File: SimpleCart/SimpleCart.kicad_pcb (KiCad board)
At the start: 2 copper layers, 90 x 56.8 mm, 9 parts, among them J1 CommanderX16Expansion Alt, U1 SST39SF040, U2 74HCT00, U3 74HCT138

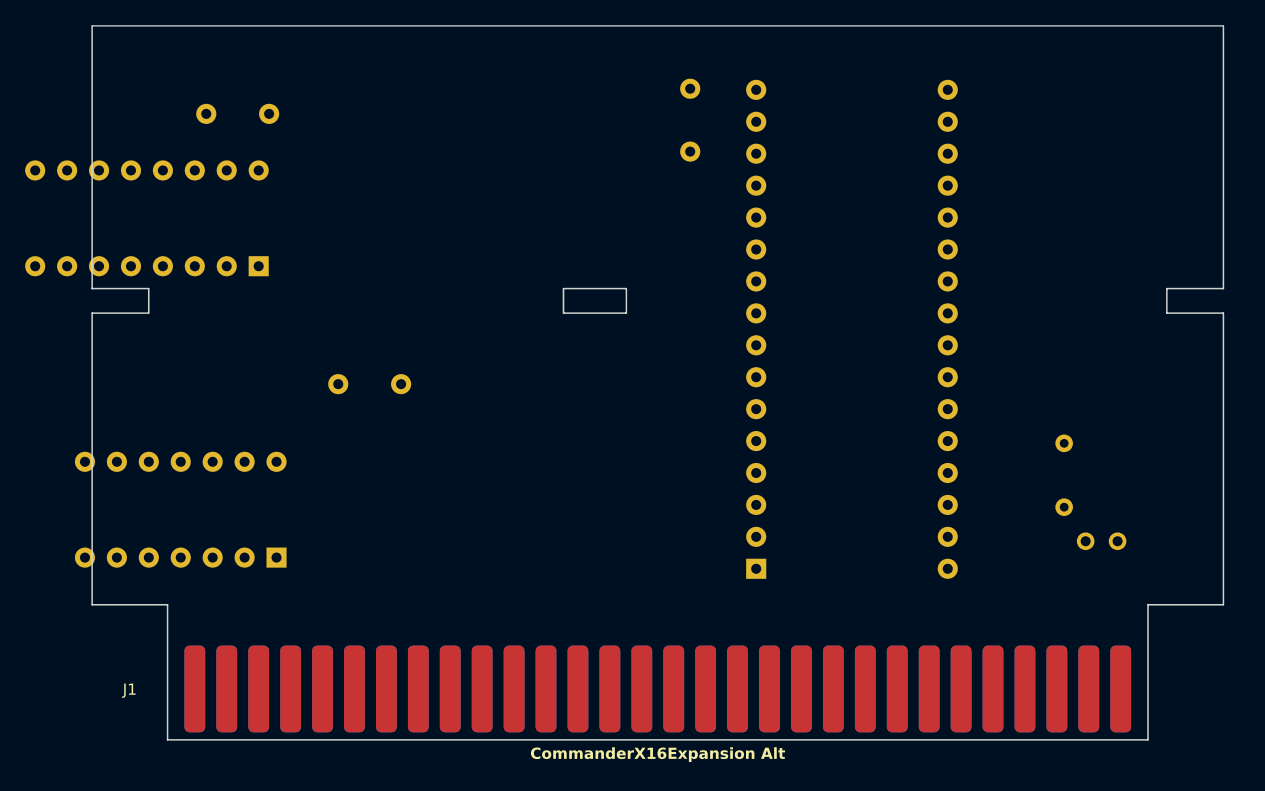
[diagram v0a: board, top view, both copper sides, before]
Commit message: BOM, fully routed
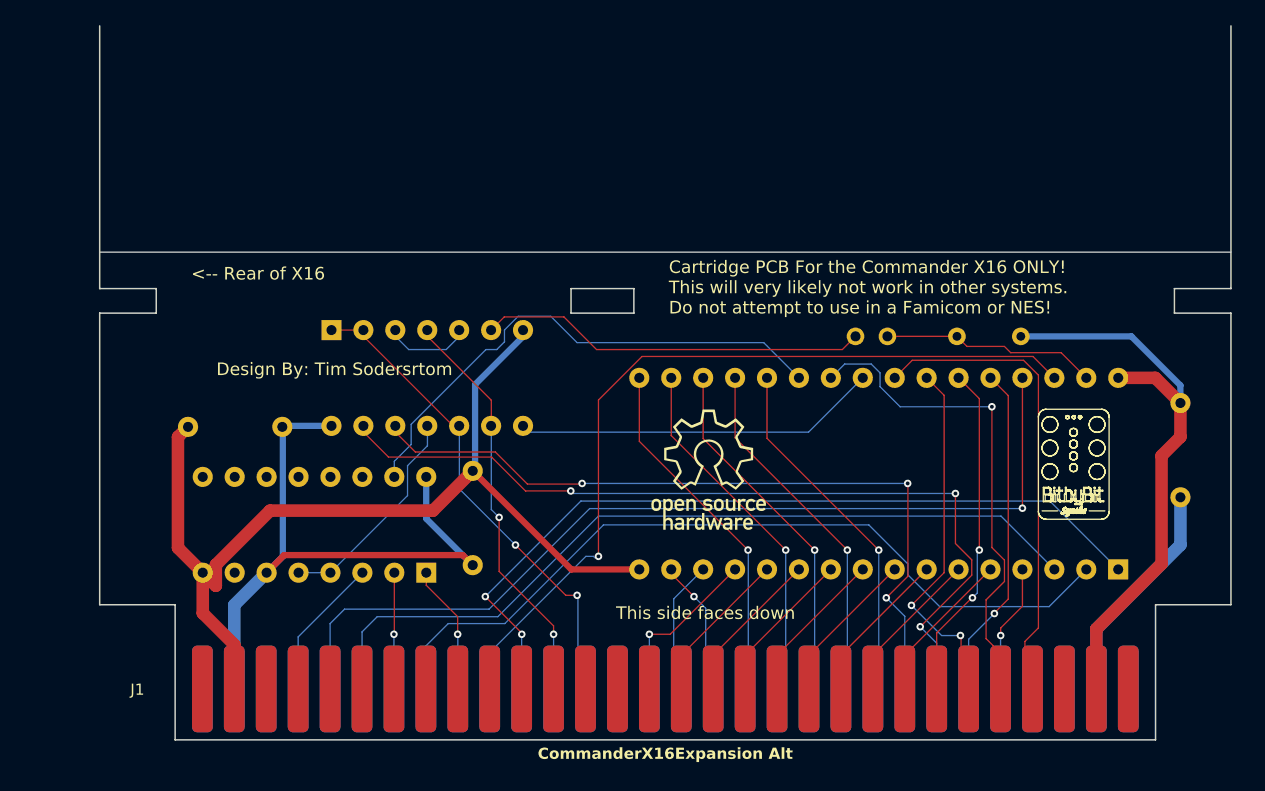
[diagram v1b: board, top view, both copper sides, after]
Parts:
- C1, C2, C3: value C -> 100nF; footprint Capacitor_THT:C_Disc_D5.0mm_W2.5mm_P5.00mm -> Capacitor_THT:C_Axial_L3.8mm_D2.6mm_P7.50mm_Horizontal
- JP1: value Jumper_2_Bridged -> WRITE EN
- U1: value SST39SF040 -> SST39SF040 (ROM)
- moved C1 50.8 mm to (134.0, 115.5), turned to 90 degrees
- moved U1 28.8 mm to (129.1, 121.2), turned to 90 degrees
- moved U3 27.8 mm to (74.0, 121.5)
- moved JP1 26.5 mm to (108.2, 102.7), turned to 0 degrees
- moved C3 24.9 mm to (62.5, 109.9)
- moved U2 18.6 mm to (66.5, 102.2), turned to -90 degrees
- moved C2 12.7 mm to (77.7, 113.4), turned to -90 degrees
- moved R1 12.0 mm to (116.2, 102.7), turned to 0 degrees
- moved J1 0.60 mm to (93.0, 130.8)
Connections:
- net Net-(J1-A0) renamed A0
- net Net-(J1-A1) renamed A1
- net Net-(J1-A10) renamed A10
- net Net-(J1-A11) renamed A11
- net Net-(J1-A12) renamed A12
- net Net-(J1-A13) renamed A13
- net Net-(J1-A2) renamed A2
- net Net-(J1-A3) renamed A3
- net Net-(J1-A4) renamed A4
- net Net-(J1-A5) renamed A5
- net Net-(J1-A6) renamed A6
- net Net-(J1-A7) renamed A7
- net Net-(J1-A8) renamed A8
- net Net-(J1-A9) renamed A9
- net Net-(J1-D0) renamed D0
- net Net-(J1-D1) renamed D1
- net Net-(J1-D2) renamed D2
- net Net-(J1-D3) renamed D3
- net Net-(J1-D4) renamed D4
- net Net-(J1-D5) renamed D5
- net Net-(J1-D6) renamed D6
- net Net-(J1-D7) renamed D7
- net Net-(J1-ROMB0) renamed ROMB0
- net Net-(J1-ROMB1) renamed ROMB1
- net Net-(J1-ROMB2) renamed ROMB2
- net Net-(J1-ROMB3) renamed ROMB3
- net Net-(J1-ROMB4) renamed ROMB4
- U3 pad 14: unconnected-(U3-~{Y1}-Pad14) -> !RAMBEN
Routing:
- net +5V: track 0.00 -> 99.0 mm
- net GND: track 0.00 -> 96.6 mm
- net ROMB0: track 0.00 -> 73.8 mm, vias 0 -> 1
- net Net-(J1-A14): track 0.00 -> 67.6 mm, vias 0 -> 3
- net ROMB3: track 0.00 -> 65.9 mm, vias 0 -> 1
- net ROMB1: track 0.00 -> 64.6 mm
- net ROMB2: track 0.00 -> 64.4 mm
- net ROMB4: track 0.00 -> 63.7 mm, vias 0 -> 2
- net Net-(J1-A15): track 0.00 -> 60.2 mm, vias 0 -> 3
- net !ROMBEN: track 0.00 -> 41.7 mm
- net A10: track 0.00 -> 39.0 mm, vias 0 -> 1
- net Net-(J1-RWB): track 0.00 -> 38.4 mm, vias 0 -> 2
- net A11: track 0.00 -> 37.9 mm
- net Net-(J1-PHI2): track 0.00 -> 32.2 mm, vias 0 -> 2
- net !MEMWE: track 0.00 -> 30.9 mm
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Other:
- board text added: "<-- Rear of X16"
- board text added: "Cartridge PCB For the Commander X16 ONLY! This will very likely not work in other systems. Do not attempt to use in a Famicom or NES!"
- board text added: "Design By: Tim Sodersrtom"
- board text added: "Rear of X16 --->"
- board text added: "This side faces down"
- board text added: "This side faces up"
